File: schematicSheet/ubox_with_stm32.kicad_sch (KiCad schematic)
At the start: 14 parts, among them U3 SAM-M10Q-00B

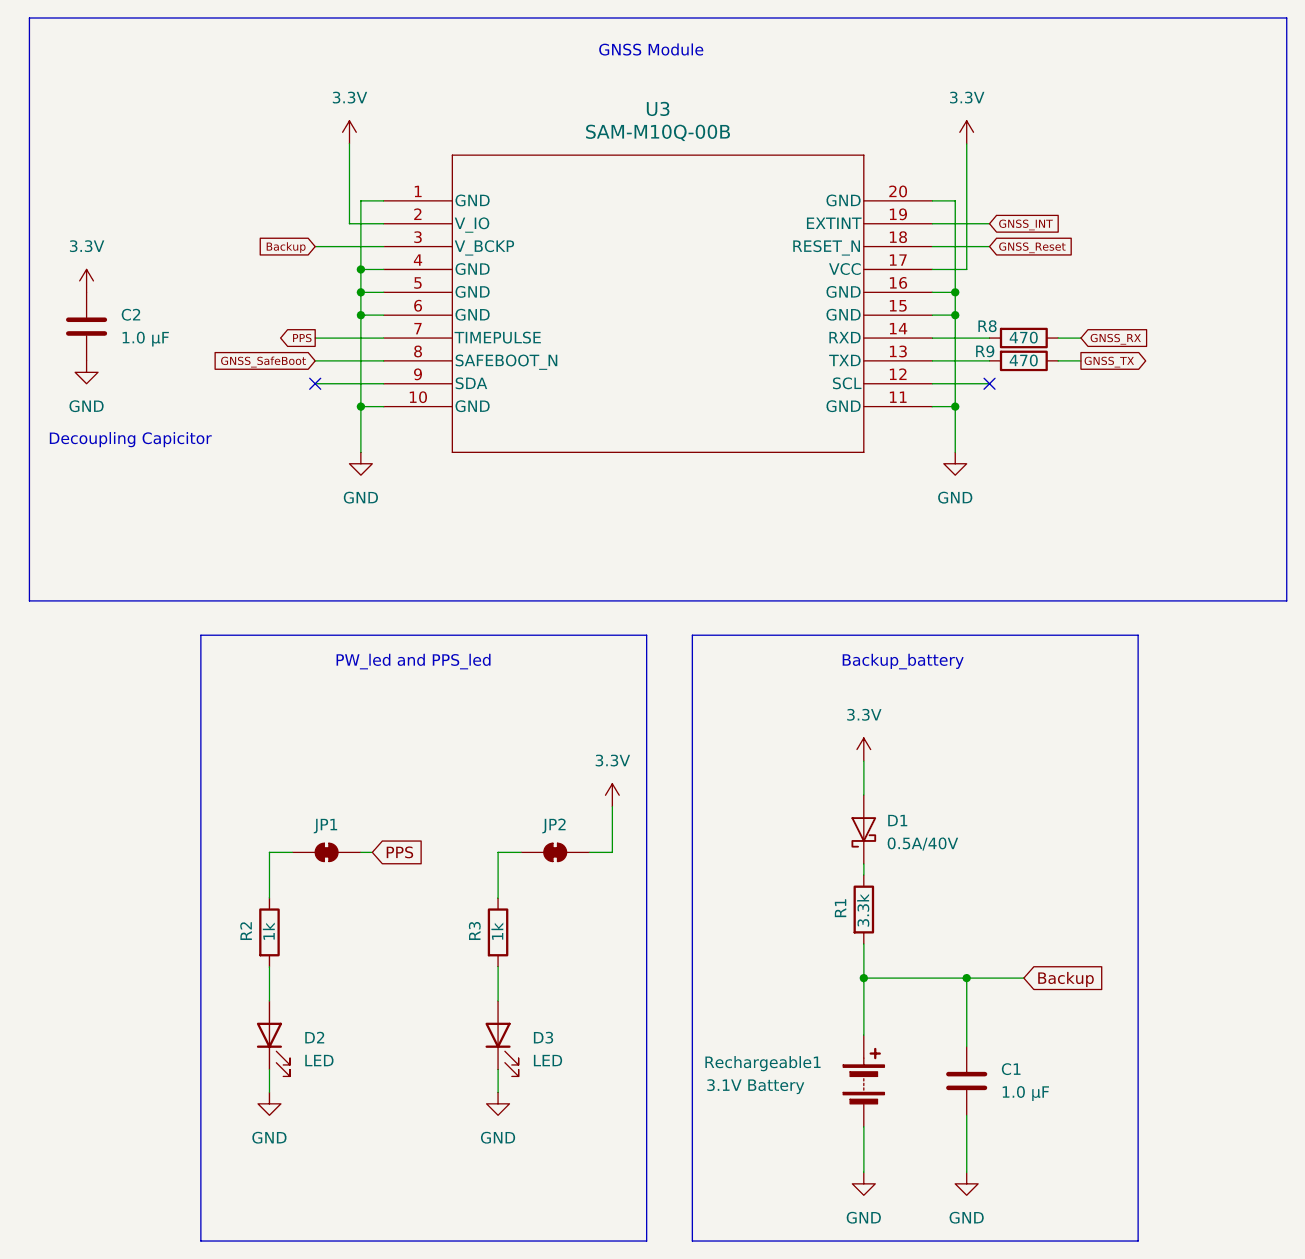
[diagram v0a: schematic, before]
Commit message: Arranged pin
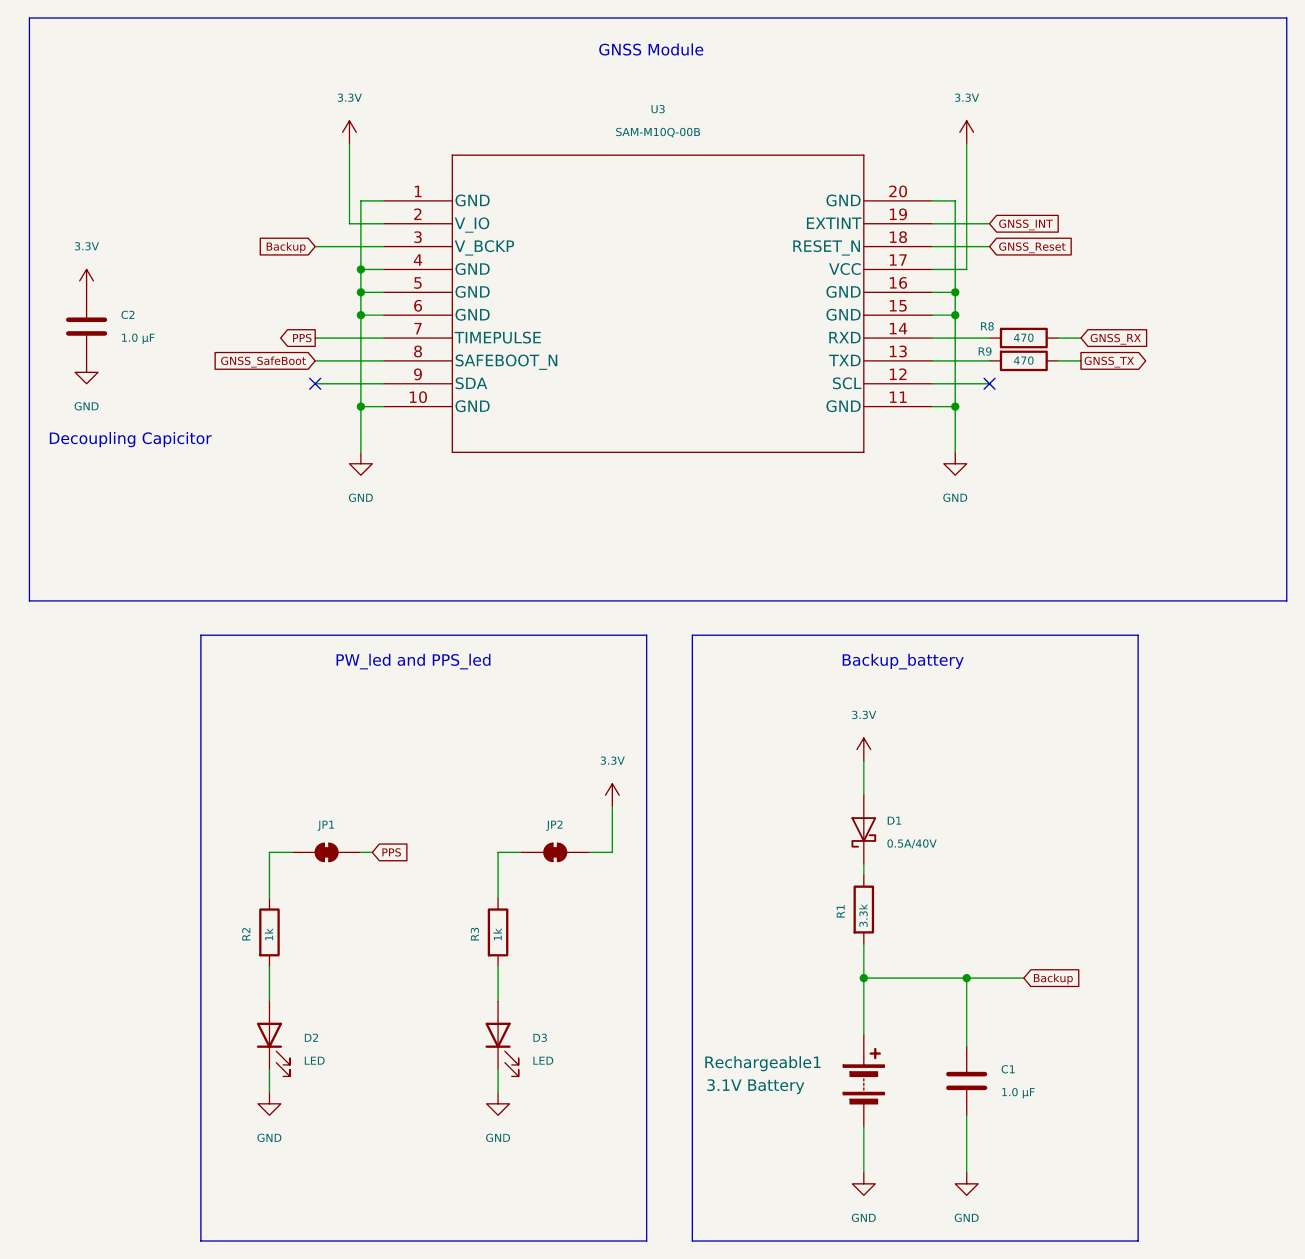
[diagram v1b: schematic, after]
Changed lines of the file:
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@@
 		(effects
 			(font
-				(size 1.27 1.27)
+				(size 0.889 0.889)
 			)
 			(justify left)
@@
 		(effects
 			(font
-				(size 1.27 1.27)
+				(size 0.889 0.889)
 			)
 			(justify left)
@@
 			(effects
 				(font
-					(size 1.27 1.27)
+					(size 0.889 0.889)
 				)
 				(justify left)
@@
 			(effects
 				(font
-					(size 1.27 1.27)
+					(size 0.889 0.889)
 				)
 				(justify left)
@@
 			(effects
 				(font
-					(size 1.27 1.27)
+					(size 0.889 0.889)
 				)
 			)
@@
 			(effects
 				(font
-					(size 1.27 1.27)
+					(size 0.889 0.889)
 				)
 				(justify left)
@@
 			(effects
 				(font
-					(size 1.27 1.27)
+					(size 0.889 0.889)
 				)
 				(justify left)
@@
 			(effects
 				(font
-					(size 1.27 1.27)
+					(size 0.889 0.889)
 				)
 			)
@@
 			(effects
 				(font
-					(size 1.27 1.27)
+					(size 0.889 0.889)
 				)
 			)
@@
 			(effects
 				(font
-					(size 1.27 1.27)
+					(size 0.889 0.889)
 				)
 			)
@@
 			(effects
 				(font
-					(size 1.27 1.27)
+					(size 0.889 0.889)
 				)
 			)
@@
 			(effects
 				(font
-					(size 1.27 1.27)
+					(size 0.889 0.889)
 				)
 				(justify right)
@@
 			(effects
 				(font
-					(size 1.27 1.27)
+					(size 0.889 0.889)
 				)
 				(justify right)
@@
 			(effects
 				(font
-					(size 1.27 1.27)
+					(size 0.889 0.889)
 				)
 				(justify right)
@@
 			(effects
 				(font
-					(size 1.27 1.27)
+					(size 0.889 0.889)
 				)
 				(justify right)
@@
 			(effects
 				(font
-					(size 1.27 1.27)
+					(size 0.889 0.889)
 				)
 			)
@@
 			(effects
 				(font
-					(size 1.27 1.27)
+					(size 0.889 0.889)
 				)
 			)
@@
 			(effects
 				(font
-					(size 1.27 1.27)
+					(size 0.889 0.889)
 				)
 			)
@@
 			(effects
 				(font
-					(size 1.27 1.27)
+					(size 0.889 0.889)
 				)
 			)
@@
 			(effects
 				(font
-					(size 1.27 1.27)
+					(size 0.889 0.889)
 				)
 				(justify left)
@@
 			(effects
 				(font
-					(size 1.27 1.27)
+					(size 0.889 0.889)
 				)
 				(justify left)
@@
 			(effects
 				(font
-					(size 1.27 1.27)
+					(size 0.889 0.889)
 				)
 			)
@@
 			(effects
 				(font
-					(size 1.27 1.27)
+					(size 0.889 0.889)
 				)
 			)
@@
 			(effects
 				(font
-					(size 1.27 1.27)
+					(size 0.889 0.889)
 				)
 				(justify left)
@@
 			(effects
 				(font
-					(size 1.27 1.27)
+					(size 0.889 0.889)
 				)
 				(justify left)
@@
 			(effects
 				(font
-					(size 1.27 1.27)
+					(size 0.889 0.889)
 				)
 			)
@@
 			(effects
 				(font
-					(size 1.27 1.27)
+					(size 0.889 0.889)
 				)
 			)
@@
 			(effects
 				(font
-					(size 1.524 1.524)
+					(size 0.889 0.889)
 				)
 			)
@@
 			(effects
 				(font
-					(size 1.524 1.524)
+					(size 0.889 0.889)
 				)
 			)
@@
 			(effects
 				(font
-					(size 1.27 1.27)
+					(size 0.889 0.889)
 				)
 				(justify right)
@@
 			(effects
 				(font
-					(size 1.27 1.27)
+					(size 0.889 0.889)
 				)
 				(justify right)
@@
 			(effects
 				(font
-					(size 1.27 1.27)
+					(size 0.889 0.889)
 				)
 			)
@@
 			(effects
 				(font
-					(size 1.27 1.27)
+					(size 0.889 0.889)
 				)
 			)
@@
 			(effects
 				(font
-					(size 1.27 1.27)
+					(size 0.889 0.889)
 				)
 			)
@@
 			(effects
 				(font
-					(size 1.27 1.27)
+					(size 0.889 0.889)
 				)
 			)
@@
 			(effects
 				(font
-					(size 1.27 1.27)
+					(size 0.889 0.889)
 				)
 			)
@@
 			(effects
 				(font
-					(size 1.27 1.27)
+					(size 0.889 0.889)
 				)
 				(justify left)
@@
 			(effects
 				(font
-					(size 1.27 1.27)
+					(size 0.889 0.889)
 				)
 				(justify left)

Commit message: update
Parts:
- C1, C2: footprint Capacitor_SMD:C_0805_2012Metric -> Capacitor_SMD:C_0402_1005Metric
- R1, R2, R3, R8, R9: footprint Resistor_SMD:R_0805_2012Metric -> Resistor_SMD:R_0402_1005Metric
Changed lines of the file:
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@@
 			)
 		)
-		(property "Footprint" "Resistor_SMD:R_0805_2012Metric"
+		(property "Footprint" "Resistor_SMD:R_0402_1005Metric"
 			(at 117.602 124.46 90)
 			(effects
@@
 			)
 		)
-		(property "Footprint" "Capacitor_SMD:C_0805_2012Metric"
+		(property "Footprint" "Capacitor_SMD:C_0402_1005Metric"
 			(at 100.0252 60.96 0)
 			(effects
@@
 			)
 		)
-		(property "Footprint" "Resistor_SMD:R_0805_2012Metric"
+		(property "Footprint" "Resistor_SMD:R_0402_1005Metric"
 			(at 203.2 59.182 90)
 			(effects
@@
 			)
 		)
-		(property "Footprint" "Capacitor_SMD:C_0805_2012Metric"
+		(property "Footprint" "Capacitor_SMD:C_0402_1005Metric"
 			(at 197.8152 144.78 0)
 			(effects
@@
 			)
 		)
-		(property "Footprint" "Resistor_SMD:R_0805_2012Metric"
+		(property "Footprint" "Resistor_SMD:R_0402_1005Metric"
 			(at 203.2 56.642 90)
 			(effects
@@
 			)
 		)
-		(property "Footprint" "Resistor_SMD:R_0805_2012Metric"
+		(property "Footprint" "Resistor_SMD:R_0402_1005Metric"
 			(at 143.002 124.46 90)
 			(effects
@@
 			)
 		)
-		(property "Footprint" "Resistor_SMD:R_0805_2012Metric"
+		(property "Footprint" "Resistor_SMD:R_0402_1005Metric"
 			(at 183.642 121.92 90)
 			(effects
